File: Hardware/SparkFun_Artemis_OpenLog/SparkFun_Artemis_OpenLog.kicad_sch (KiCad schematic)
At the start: 88 parts, among them J1 USB_C_Receptacle, J2 Conn_01x06, J3 SWD, J4 Conn_01x01, J5 JST_2mm_LiPo, J6 Conn_01x02, J7 Conn_01x02, J8 Qwiic_RA, J9 microSD, Q1 DMG2305UX, SW1 SMD_4.6x2.8mm_h2.5mm, U1 MAX810TTRG, U2 CH340E, U3 Artemis Module, U4 MCP73831, U5 AP2112K-3.3, U6 BNO086, U7 AP2112K-3.3, Y1 32.768kHz, Y2 32.768kHz

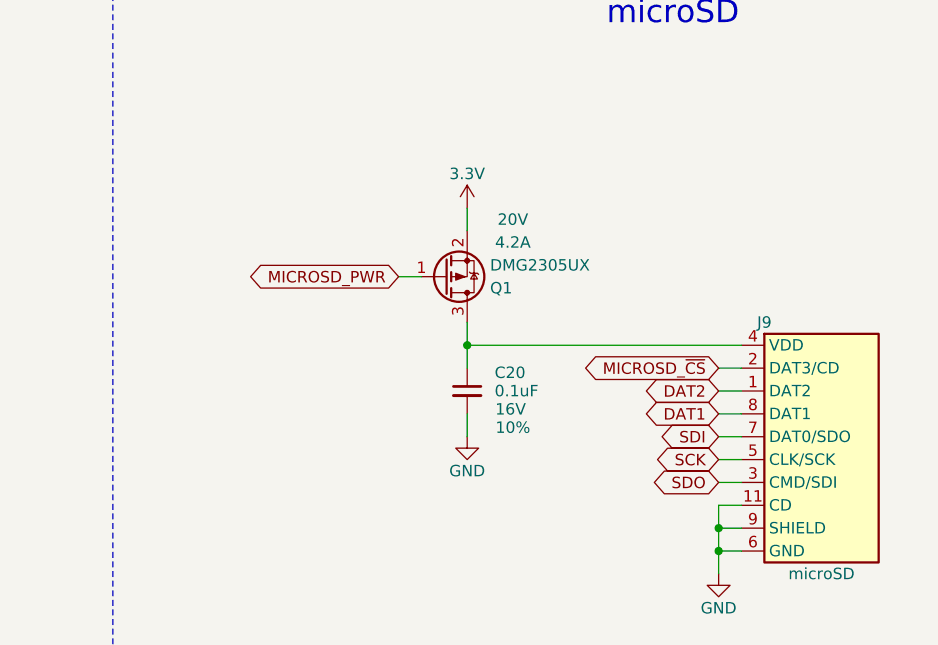
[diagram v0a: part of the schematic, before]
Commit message: Save before switch for IMU update
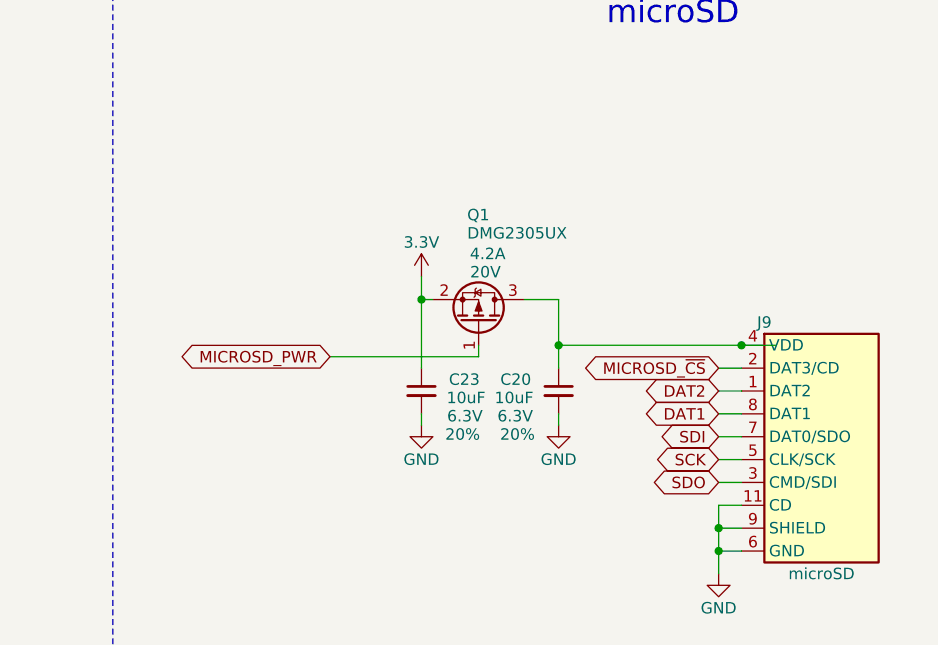
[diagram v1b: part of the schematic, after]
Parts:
- added C23: 10uF, SparkFun-Capacitor:C_0402_1005Metric, symbol SparkFun-Capacitor:10uF_0402_6.3V_20%
- C20: value 0.1uF -> 10uF; symbol SparkFun-Capacitor:0.1uF_0402_16V_10% -> SparkFun-Capacitor:10uF_0402_6.3V_20%; PROD_ID CAP-25565 -> CAP-14848; Tolerance 10% -> 20%; Voltage 16V -> 6.3V
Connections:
- net 3.3V: now also C23.1
- net GND: now also C23.2
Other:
- moved on the sheet: C20, Q1
